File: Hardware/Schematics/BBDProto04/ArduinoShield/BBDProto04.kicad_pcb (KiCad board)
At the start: 2 copper layers, 91.4 x 106.7 mm, 34 parts, among them P1 Power, P11 CONN_02X08, P12 CONN_02X08, P13 CONN_02X08, P14 CONN_02X08, P15 CONN_02X08, P16 CONN_02X08, P17 CONN_02X08, P18 CONN_02X08, P2 Analog, P3 Digital, P4 Digital, P5 CONN_1, P6 CONN_1, P7 CONN_1, P8 CONN_1, P9 USBASP, Q1 Q_NPN_BCE, SW1 SW_PUSH, U1 ATTINY861-20SU, U10 CD74HC4067, U11 CD74HC4067, U12 CD74HC4067, U13 CD74HC4067, U14 CD74HC4067, U15 CD74HC4067, U16 CD74HC4067, U17 CD74HC4067, U18 CD74HC4067, U2 LTC1864, U3 MCP4822

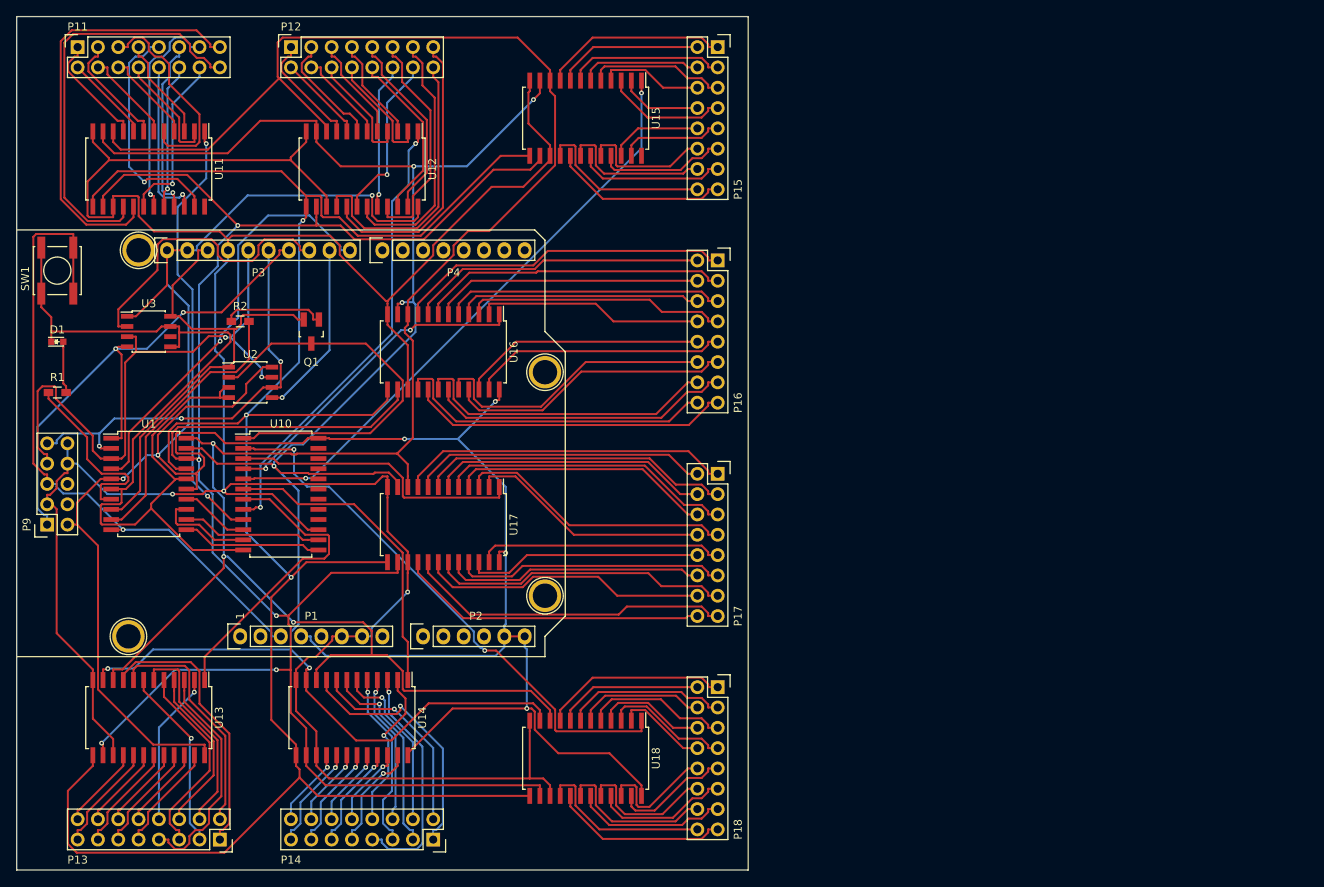
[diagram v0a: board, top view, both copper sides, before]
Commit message: Proto #4 - Rev A
Proto #4 - Rev A
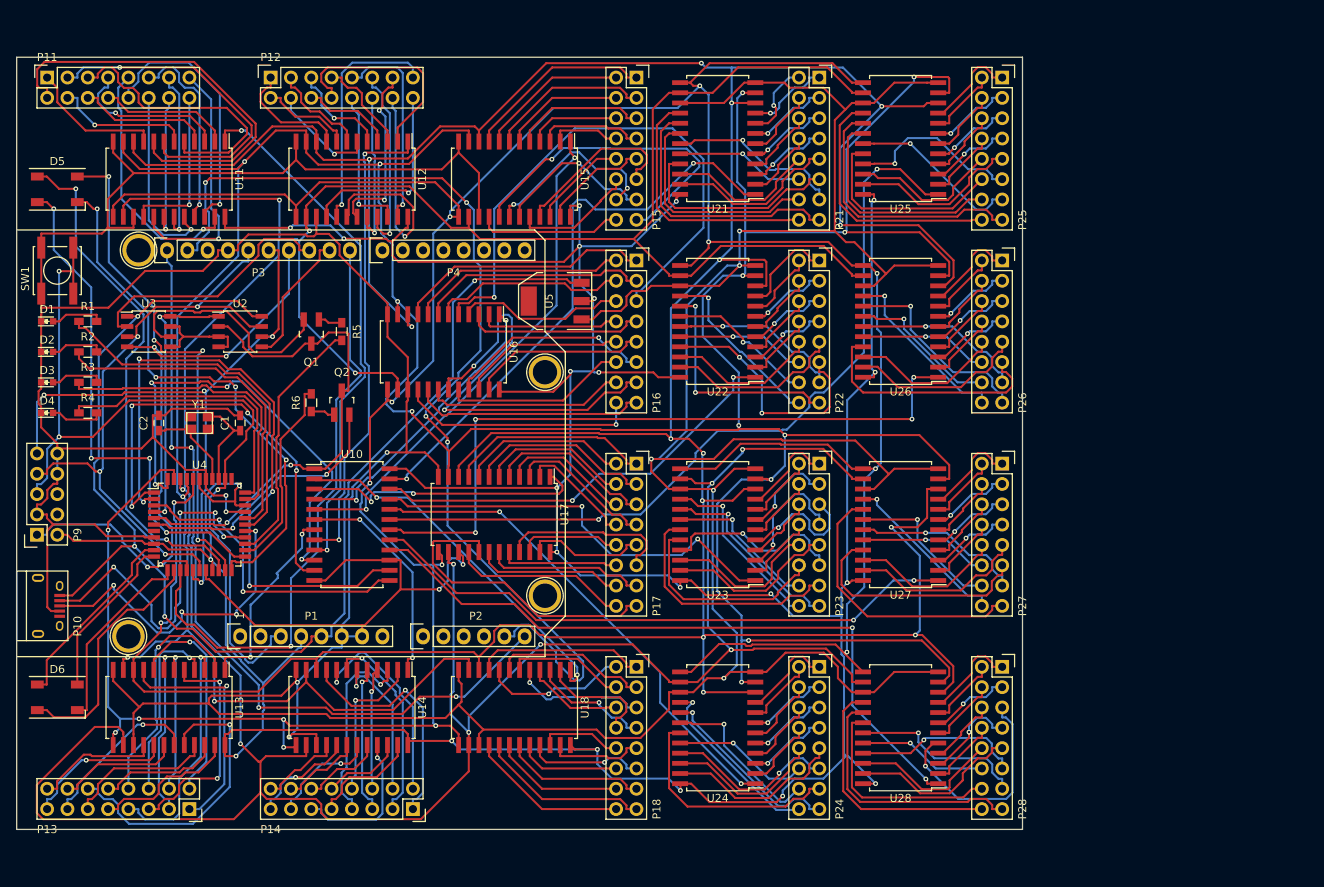
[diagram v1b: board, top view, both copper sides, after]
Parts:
- removed U1: ATTINY861-20SU, Housings_SOIC:SOIC-20_7.5x12.8mm_Pitch1.27mm
- added C1: 12pF, Capacitors_SMD:C_0603_HandSoldering, F.Cu at (56.4, 90.8)
- added C2: 12pF, Capacitors_SMD:C_0603_HandSoldering, F.Cu at (46.2, 90.8)
- added D2: LED, LEDs:LED_0603, F.Cu at (32.3, 81.9)
- added D3: LED, LEDs:LED_0603, F.Cu at (32.3, 85.7)
- added D4: LED, LEDs:LED_0603, F.Cu at (32.3, 89.5)
- added D5: LED_RCBG, LEDs:LED_WS2812B-PLCC4, F.Cu at (33.5, 61.6)
- added D6: LED_RCBG, LEDs:LED_WS2812B-PLCC4, F.Cu at (33.5, 125.1)
- added P10: USB_B, Connect:USB_Micro-B, F.Cu at (32.3, 113.7)
- added P21: CONN_02X08, Socket_Strips:Socket_Strip_Straight_2x08, F.Cu at (128.8, 47.6)
- added P22: CONN_02X08, Socket_Strips:Socket_Strip_Straight_2x08, F.Cu at (128.8, 70.5)
- added P23: CONN_02X08, Socket_Strips:Socket_Strip_Straight_2x08, F.Cu at (128.8, 95.9)
- added P24: CONN_02X08, Socket_Strips:Socket_Strip_Straight_2x08, F.Cu at (128.8, 121.3)
- added P25: CONN_02X08, Socket_Strips:Socket_Strip_Straight_2x08, F.Cu at (151.6, 47.6)
- added P26: CONN_02X08, Socket_Strips:Socket_Strip_Straight_2x08, F.Cu at (151.6, 70.5)
- added P27: CONN_02X08, Socket_Strips:Socket_Strip_Straight_2x08, F.Cu at (151.6, 95.9)
- added P28: CONN_02X08, Socket_Strips:Socket_Strip_Straight_2x08, F.Cu at (151.6, 121.3)
- added Q2: Q_NPN_BCE, TO_SOT_Packages_SMD:SOT-23_Handsoldering, F.Cu at (69.1, 88.3)
- added R3: 1k, Resistors_SMD:R_0603_HandSoldering, F.Cu at (37.3, 85.7)
- added R4: 1k, Resistors_SMD:R_0603_HandSoldering, F.Cu at (37.3, 89.5)
- added R5: 1k, Resistors_SMD:R_0603_HandSoldering, F.Cu at (69.1, 79.4)
- added R6: 1k, Resistors_SMD:R_0603_HandSoldering, F.Cu at (65.3, 88.3)
- added U21: CD74HC4067, Housings_SOIC:SOIC-24_7.5x15.4mm_Pitch1.27mm, F.Cu at (116.1, 55.2)
- added U22: CD74HC4067, Housings_SOIC:SOIC-24_7.5x15.4mm_Pitch1.27mm, F.Cu at (116.1, 78.1)
- added U23: CD74HC4067, Housings_SOIC:SOIC-24_7.5x15.4mm_Pitch1.27mm, F.Cu at (116.1, 103.5)
- added U24: CD74HC4067, Housings_SOIC:SOIC-24_7.5x15.4mm_Pitch1.27mm, F.Cu at (116.1, 128.9)
- added U25: CD74HC4067, Housings_SOIC:SOIC-24_7.5x15.4mm_Pitch1.27mm, F.Cu at (138.9, 55.2)
- added U26: CD74HC4067, Housings_SOIC:SOIC-24_7.5x15.4mm_Pitch1.27mm, F.Cu at (138.9, 78.1)
- added U27: CD74HC4067, Housings_SOIC:SOIC-24_7.5x15.4mm_Pitch1.27mm, F.Cu at (138.9, 103.5)
- added U28: CD74HC4067, Housings_SOIC:SOIC-24_7.5x15.4mm_Pitch1.27mm, F.Cu at (138.9, 128.9)
- added U4: ATXMEGA128A4U-AU, Housings_QFP:TQFP-44_10x10mm_Pitch0.8mm, F.Cu at (51.3, 103.5)
- added U5: LD1117AS33TR, TO_SOT_Packages_SMD:SOT-223, F.Cu at (95.8, 75.6)
- added Y1: Crystal, Crystals:crystal_FA238-TSX3225, F.Cu at (51.3, 90.8)
- moved R2 19.4 mm to (37.3, 81.9)
- moved U15 11.7 mm to (90.7, 60.3)
- moved U18 10.9 mm to (90.7, 126.4)
- moved P15 10.9 mm to (105.9, 47.6)
- moved P18 10.5 mm to (105.9, 121.3)
- moved P17 10.2 mm to (105.9, 95.9)
- moved P16 10.2 mm to (105.9, 70.5)
- moved R1 9.67 mm to (37.3, 78.1)
- moved U10 9.67 mm to (70.4, 103.5)
- moved U17 6.48 mm to (88.1, 102.2)
- moved U2 6.48 mm to (56.4, 79.4)
- moved P13 5.39 mm to (50.0, 139.1)
- moved P11 5.39 mm to (32.3, 47.6)
- moved P14 4.58 mm to (78.0, 139.1)
- moved P12 4.58 mm to (60.2, 47.6)
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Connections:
- net /Reset renamed /RESET
- net Net-(Q1-Pad3) renamed /MULTIPLEXER-INPUT
- net Net-(U1-Pad17) renamed /MULTIPLEXER-S3
- net Net-(U1-Pad18) renamed /MULTIPLEXER-S2
- net Net-(U1-Pad19) renamed /MULTIPLEXER-S1
- net Net-(U1-Pad20) renamed /MULTIPLEXER-S0-LSB
- D1 pad 1: Net-(D1-Pad1) -> GND
- P2 pad 5: /+3.3V -> /A4(SDA)
- P2 pad 6: /+3.3V -> /A5(SCL)
- P3 pad 1: /+3.3V -> /A5(SCL)
- P3 pad 2: /+3.3V -> /A4(SDA)
- Q1 pad 2: /AREF -> /DAC-MULTIPLEXER-OUTPUT
- R2 pad 1: Net-(Q1-Pad1) -> Net-(R2-Pad1)
- SW1 pad 1: Net-(D1-Pad1) -> GND
- U10 pad 10: Net-(U1-Pad14) -> /MULTIPLEXER-S4
- U10 pad 11: Net-(U1-Pad13) -> /MULTIPLEXER-S5
- U10 pad 12: Net-(D1-Pad1) -> GND
- U10 pad 13: Net-(U1-Pad11) -> /MULTIPLEXER-S7-MSB
- U10 pad 14: Net-(U1-Pad12) -> /MULTIPLEXER-S6
- U11 pad 24: Net-(U11-Pad24) -> /+3.3V
- U15 pad 24: Net-(U15-Pad24) -> /+3.3V
- U2 pad 1: /AREF -> /ADC-VREF
- U2 pad 3: Net-(D1-Pad1) -> Net-(U2-Pad3)
- U2 pad 4: Net-(D1-Pad1) -> Net-(U2-Pad3)
- U2 pad 8: /+3.3V -> /+5.0V
- U3 pad 1: /+3.3V -> /+5.0V
- U3 pad 5: Net-(D1-Pad1) -> Net-(U2-Pad3)
- U3 pad 6: Net-(U3-Pad6) -> /DAC-MULTIPLEXER-OUTPUT
- U3 pad 7: Net-(D1-Pad1) -> Net-(U2-Pad3)
- U3 pad 8: /AREF -> /ADC-VREF
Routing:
- net GND: track 366.6 -> 756.4 mm, vias 3 -> 12
- net /MULTIPLEXER-S1: track 237.8 -> 481.9 mm, vias 6 -> 16
- net /MULTIPLEXER-S2: track 258.7 -> 493.2 mm, vias 5 -> 11
- net /MULTIPLEXER-S0-LSB: track 265.2 -> 493.5 mm, vias 3 -> 16
- net /MULTIPLEXER-S3: track 271.5 -> 436.1 mm, vias 3 -> 15
- net /+5.0V: track 0.00 -> 163.1 mm, vias 0 -> 4
- net /+3.3V: track 324.9 -> 467.9 mm, vias 7 -> 23
- net /A4(SDA): track 0.00 -> 130.2 mm, vias 0 -> 4
- net Net-(D1-Pad1): track 119.3 -> 0.00 mm
- net Net-(U10-Pad19): track 0.00 -> 101.6 mm, vias 0 -> 2
- net /A5(SCL): track 0.00 -> 101.1 mm, vias 0 -> 4
- net Net-(U10-Pad18): track 0.00 -> 88.0 mm, vias 0 -> 4
- net Net-(U10-Pad16): track 0.00 -> 86.6 mm, vias 0 -> 2
- net /MULTIPLEXER-S6: track 0.00 -> 81.4 mm, vias 0 -> 4
- net Net-(U10-Pad17): track 0.00 -> 74.8 mm, vias 0 -> 2
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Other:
- board size 91.4 x 106.7 mm -> 125.7 x 96.5 mm
- net class Default: clearance 0.2 -> 0.254; trace_width 0.25 -> 0.254
- rule trace_clearance: 0.2 -> 0.254
- board text added: "Bio Balance Detector #4 Rev. A (2016-05-03) Andras Fuchs (andras.fuchs@gmail.com)"
- board text removed: "Bio Balance Detector Rev. B (2016-04-07) Andras Fuchs (andras.fuchs@gmail.com)"

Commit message: BBDProto04 ArduinoShield RevC
BBDProto04 ArduinoShield RevC
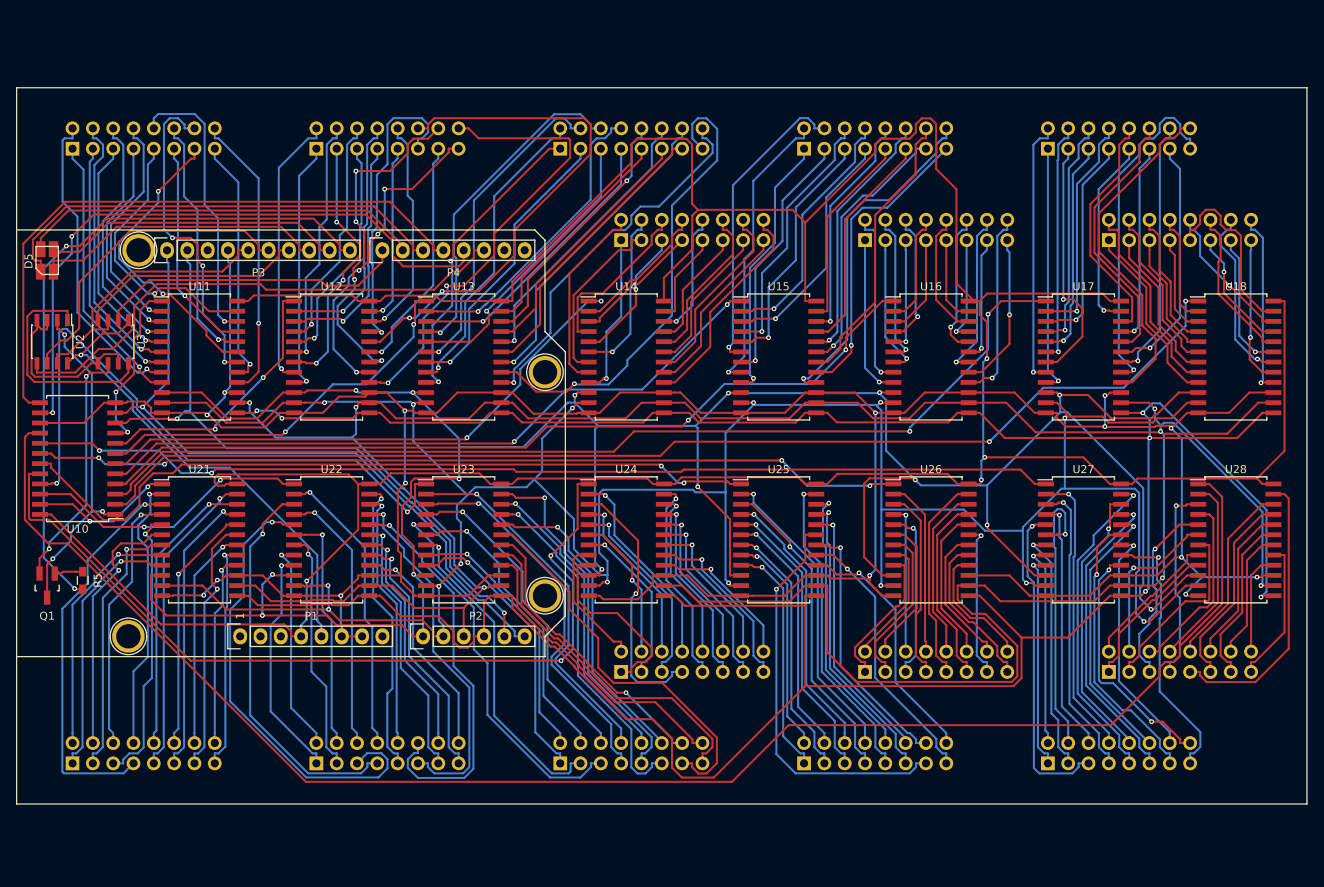
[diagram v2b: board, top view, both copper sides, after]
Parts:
- removed C1, C2: 12pF, Capacitors_SMD:C_0603_HandSoldering
- removed D1, D2, D3, D4: LED, LEDs:LED_0603
- removed D6: LED_RCBG, LEDs:LED_WS2812B-PLCC4
- removed P10: USB_B, Connect:USB_Micro-B
- removed P9: USBASP, Socket_Strips:Socket_Strip_Straight_2x05
- removed Q2: Q_NPN_BCE, TO_SOT_Packages_SMD:SOT-23_Handsoldering
- removed R1, R2, R3, R4, R6: 1k, Resistors_SMD:R_0603_HandSoldering
- removed SW1: SW_PUSH, Buttons_Switches_SMD:SW_SPST_EVPBF
- removed U4: ATXMEGA128A4U-AU, Housings_QFP:TQFP-44_10x10mm_Pitch0.8mm
- removed U5: LD1117AS33TR, TO_SOT_Packages_SMD:SOT-223
- removed Y1: Crystal, Crystals:crystal_FA238-TSX3225
- D5: footprint LEDs:LED_WS2812B-PLCC4 -> OptoSupply_LEDs:LED_3528-PLCC4
- P11, P12, P13, P14, P15, P16, P17, P18, P21, P22, P23, P24, P25, P26, P27, P28: moved to B.Cu
- moved P21 126.7 mm to (35.4, 133.3), turned to 0 degrees
- moved U18 100.3 mm to (180.8, 82.5), turned to 0 degrees
- moved P13 94.7 mm to (96.4, 56.5), turned to 0 degrees
- moved P25 89.2 mm to (126.9, 133.3), turned to 0 degrees
- moved P22 88.9 mm to (65.9, 133.3), turned to 0 degrees
- moved U21 81.9 mm to (51.3, 105.4), turned to 0 degrees
- moved P18 79.6 mm to (165.0, 67.9), turned to 0 degrees
- moved U17 76.2 mm to (161.8, 82.5), turned to 0 degrees
- moved P14 75.7 mm to (104.0, 67.9), turned to 0 degrees
- moved P17 64.8 mm to (157.4, 56.5), turned to 0 degrees
- moved U16 61.0 mm to (142.7, 82.5), turned to 0 degrees
- moved U13 57.2 mm to (84.3, 82.5), turned to 0 degrees
- moved U14 55.6 mm to (104.6, 82.5), turned to 0 degrees
- moved U22 55.4 mm to (67.8, 105.4), turned to 0 degrees
- moved P26 54.2 mm to (134.5, 121.9), turned to 0 degrees
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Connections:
- D5 pad 1: /LED-RED -> /5(**)
- D5 pad 2: /LED-POWER -> /10(**/SS)
- D5 pad 3: /LED-BLUE -> /9(**)
- D5 pad 4: /LED-GREEN -> /6(**)
- P1 pad 3: /RESET -> /Reset
- R5 pad 2: Net-(R5-Pad2) -> /8
- U10 pad 10: /MULTIPLEXER-S4 -> /A4(SDA)
- U10 pad 11: /MULTIPLEXER-S5 -> /A5(SCL)
- U10 pad 13: /MULTIPLEXER-S7-MSB -> /4
- U10 pad 14: /MULTIPLEXER-S6 -> /3(**)
- U11 pad 10: /MULTIPLEXER-S0-LSB -> /A0
- U11 pad 11: /MULTIPLEXER-S1 -> /A1
- U11 pad 13: /MULTIPLEXER-S3 -> /A3
- U11 pad 14: /MULTIPLEXER-S2 -> /A2
- U12 pad 10: /MULTIPLEXER-S0-LSB -> /A0
- U12 pad 11: /MULTIPLEXER-S1 -> /A1
- U12 pad 13: /MULTIPLEXER-S3 -> /A3
- U12 pad 14: /MULTIPLEXER-S2 -> /A2
- U13 pad 10: /MULTIPLEXER-S0-LSB -> /A0
- U13 pad 11: /MULTIPLEXER-S1 -> /A1
- U13 pad 13: /MULTIPLEXER-S3 -> /A3
- U13 pad 14: /MULTIPLEXER-S2 -> /A2
- U14 pad 10: /MULTIPLEXER-S0-LSB -> /A0
- U14 pad 11: /MULTIPLEXER-S1 -> /A1
- U14 pad 13: /MULTIPLEXER-S3 -> /A3
- U14 pad 14: /MULTIPLEXER-S2 -> /A2
- U15 pad 10: /MULTIPLEXER-S0-LSB -> /A0
- U15 pad 11: /MULTIPLEXER-S1 -> /A1
- U15 pad 13: /MULTIPLEXER-S3 -> /A3
- U15 pad 14: /MULTIPLEXER-S2 -> /A2
- U16 pad 10: /MULTIPLEXER-S0-LSB -> /A0
- U16 pad 11: /MULTIPLEXER-S1 -> /A1
- U16 pad 13: /MULTIPLEXER-S3 -> /A3
- U16 pad 14: /MULTIPLEXER-S2 -> /A2
- U17 pad 10: /MULTIPLEXER-S0-LSB -> /A0
- U17 pad 11: /MULTIPLEXER-S1 -> /A1
- U17 pad 13: /MULTIPLEXER-S3 -> /A3
- U17 pad 14: /MULTIPLEXER-S2 -> /A2
- U18 pad 10: /MULTIPLEXER-S0-LSB -> /A0
- U18 pad 11: /MULTIPLEXER-S1 -> /A1
- U18 pad 13: /MULTIPLEXER-S3 -> /A3
- U18 pad 14: /MULTIPLEXER-S2 -> /A2
- U2 pad 5: /9(**) -> /2
- U21 pad 10: /MULTIPLEXER-S0-LSB -> /A0
- U21 pad 11: /MULTIPLEXER-S1 -> /A1
- U21 pad 13: /MULTIPLEXER-S3 -> /A3
- U21 pad 14: /MULTIPLEXER-S2 -> /A2
- U22 pad 10: /MULTIPLEXER-S0-LSB -> /A0
- U22 pad 11: /MULTIPLEXER-S1 -> /A1
- U22 pad 13: /MULTIPLEXER-S3 -> /A3
- U22 pad 14: /MULTIPLEXER-S2 -> /A2
- U23 pad 10: /MULTIPLEXER-S0-LSB -> /A0
- U23 pad 11: /MULTIPLEXER-S1 -> /A1
- U23 pad 13: /MULTIPLEXER-S3 -> /A3
- U23 pad 14: /MULTIPLEXER-S2 -> /A2
- U24 pad 10: /MULTIPLEXER-S0-LSB -> /A0
- U24 pad 11: /MULTIPLEXER-S1 -> /A1
- U24 pad 13: /MULTIPLEXER-S3 -> /A3
- U24 pad 14: /MULTIPLEXER-S2 -> /A2
- U25 pad 10: /MULTIPLEXER-S0-LSB -> /A0
- U25 pad 11: /MULTIPLEXER-S1 -> /A1
- U25 pad 13: /MULTIPLEXER-S3 -> /A3
- U25 pad 14: /MULTIPLEXER-S2 -> /A2
- U26 pad 10: /MULTIPLEXER-S0-LSB -> /A0
- U26 pad 11: /MULTIPLEXER-S1 -> /A1
- U26 pad 13: /MULTIPLEXER-S3 -> /A3
- U26 pad 14: /MULTIPLEXER-S2 -> /A2
- U27 pad 10: /MULTIPLEXER-S0-LSB -> /A0
- U27 pad 11: /MULTIPLEXER-S1 -> /A1
- U27 pad 13: /MULTIPLEXER-S3 -> /A3
- U27 pad 14: /MULTIPLEXER-S2 -> /A2
- U28 pad 10: /MULTIPLEXER-S0-LSB -> /A0
- U28 pad 11: /MULTIPLEXER-S1 -> /A1
- U28 pad 13: /MULTIPLEXER-S3 -> /A3
- U28 pad 14: /MULTIPLEXER-S2 -> /A2
- U3 pad 2: /10(**/SS) -> /7
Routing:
- net /MULTIPLEXER-S0-LSB: track 493.5 -> 0.00 mm, vias 16 -> 0
- net /MULTIPLEXER-S2: track 493.2 -> 0.00 mm, vias 11 -> 0
- net /MULTIPLEXER-S1: track 481.9 -> 0.00 mm, vias 16 -> 0
- net /MULTIPLEXER-S3: track 436.1 -> 0.00 mm, vias 15 -> 0
- net /A3: track 0.00 -> 385.3 mm, vias 0 -> 6
- net /A2: track 0.00 -> 366.2 mm, vias 0 -> 7
- net /A0: track 0.00 -> 365.4 mm, vias 0 -> 15
- net /A1: track 0.00 -> 355.9 mm, vias 0 -> 15
- net GND: track 756.4 -> 406.6 mm, vias 12 -> 15
- net Net-(U10-Pad16): track 86.6 -> 203.3 mm, vias 2 -> 0
- net /RESET: track 105.7 -> 0.00 mm, vias 3 -> 0
- net Net-(U10-Pad2): track 46.4 -> 148.4 mm
- net /+5.0V: track 163.1 -> 61.0 mm, vias 4 -> 1
- net Net-(U10-Pad3): track 35.6 -> 129.6 mm
- net /MULTIPLEXER-S6: track 81.4 -> 0.00 mm, vias 4 -> 0
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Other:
- board size 125.7 x 96.5 mm -> 161.3 x 89.5 mm
- board text added: "Bio Balance Detector #4 Rev. C (2016-06-03) Andras Fuchs (andras.fuchs@gmail.com)"
- board text removed: "Bio Balance Detector #4 Rev. A (2016-05-03) Andras Fuchs (andras.fuchs@gmail.com)"
